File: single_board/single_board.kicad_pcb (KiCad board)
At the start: 4 copper layers, 118.6 x 108.9 mm, 121 parts, among them J1 SWD, J11 SPI Debug, J17 BOOTSEL, J2 USB_C_Receptacle_USB2.0_16P, J3 RST, J30 JST_GH_H, J31 JST_GH_H, J32 PB_Vertical, J33 JST_GH_H, J34 PB_Vertical, J35 JST_GH_H, J36 JST_GH_H, J37 JST_GH_H, J38 PB_Vertical, J39 PB_Vertical, J4 Conn_01x02, J40 PB_Vertical, J41 PB_Vertical, J42 PB_Vertical, J43 PB_Vertical, J44 PB_Vertical, J45 PB_Vertical, J46 PB_Vertical, J47 PB_Vertical, J48 PB_Vertical, J49 PB_Vertical, J5 Conn_01x02, J50 PB_Vertical, J6 Conn_01x02, J7 Conn_01x02, Q1 AO3401A, Q2 AO3401A, Q3 AO3401A, Q4 AO3401A, Q5 2N7002, SW1 Button, U1 AP2112K-3.3, U3 USBLC6-2SC6, U4 LSM6DSV, U5 STM32G474VBTx, Y1 FC-135

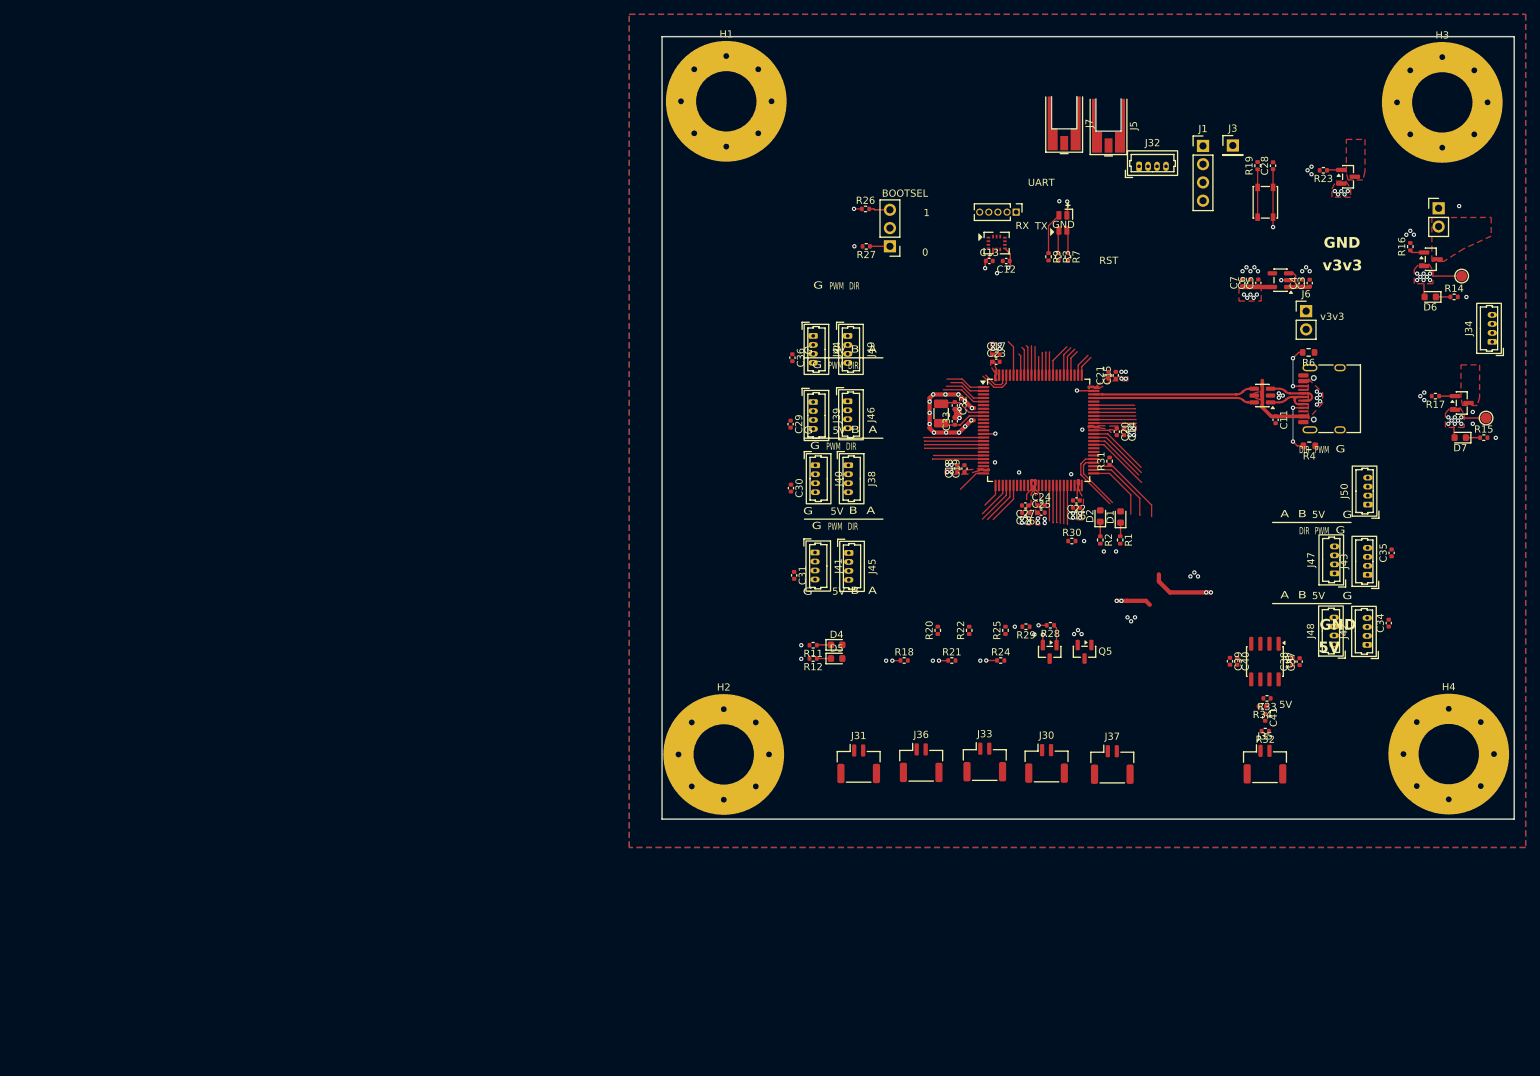
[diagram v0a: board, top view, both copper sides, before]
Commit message: PCB Layout
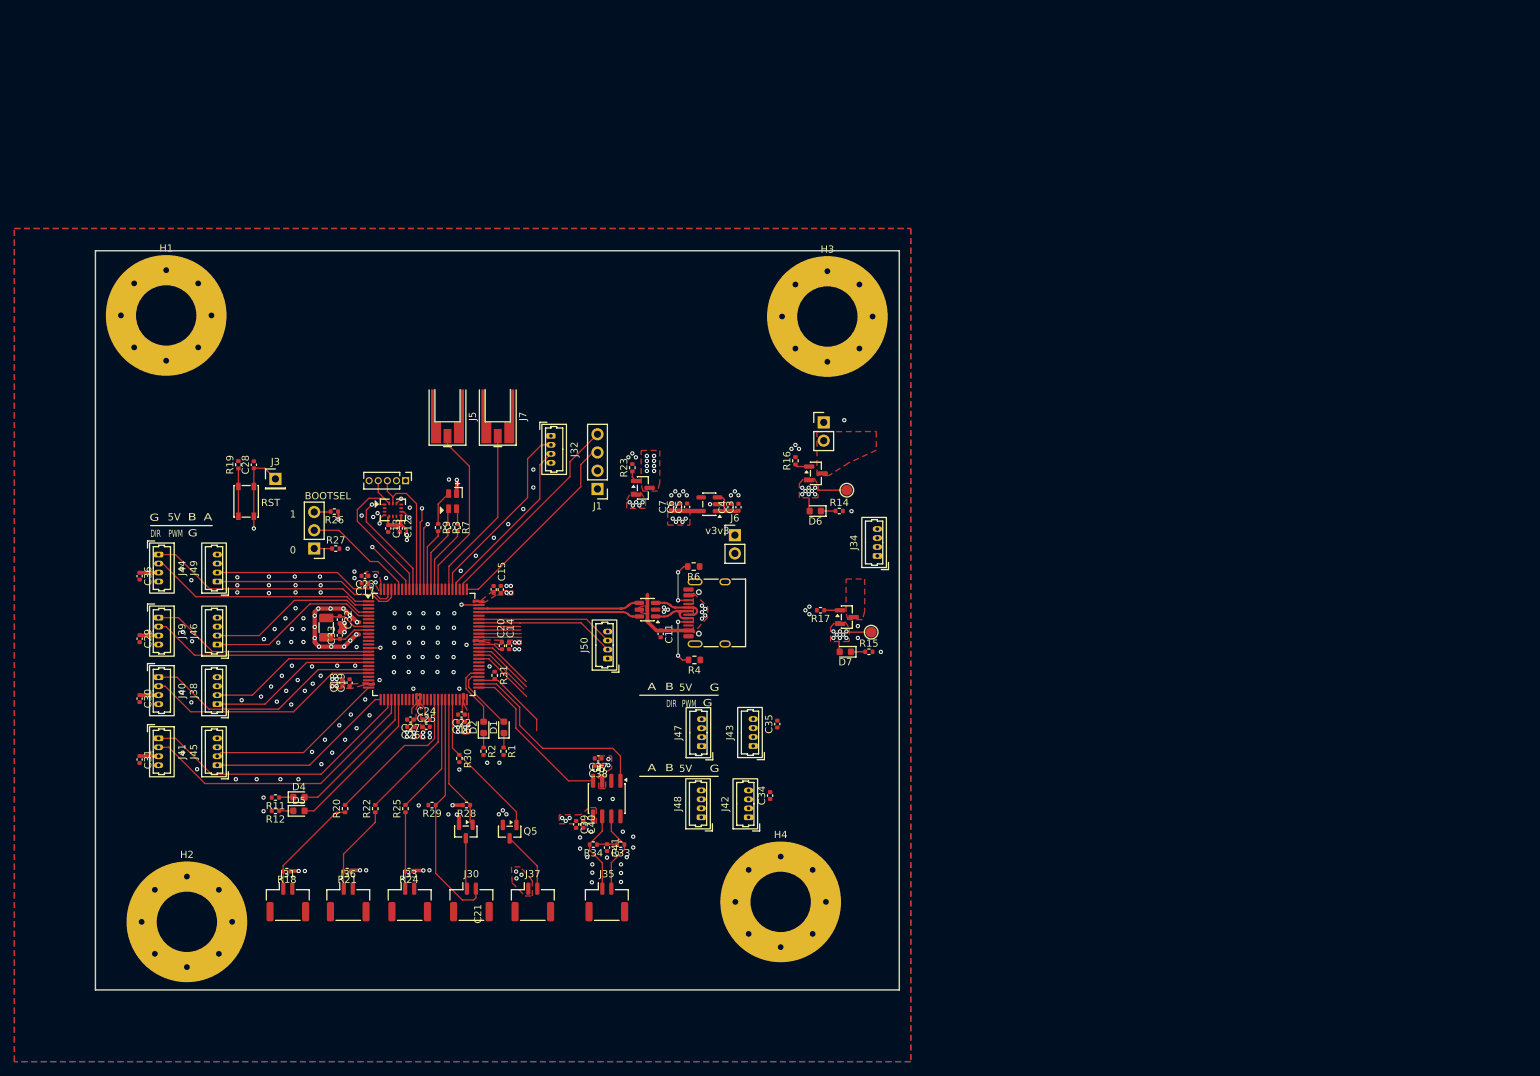
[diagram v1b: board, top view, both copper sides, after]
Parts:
- removed R32: 120, Resistor_SMD:R_0402_1005Metric
- moved C28 147.8 mm to (40.8, 118.8)
- moved R19 147.8 mm to (38.6, 118.8)
- moved SW1 147.8 mm to (39.7, 123.9)
- moved J3 141.1 mm to (43.8, 120.8)
- moved J50 107.9 mm to (90.0, 145.8)
- moved Q3 107.3 mm to (94.9, 122.0)
- moved R23 104.7 mm to (93.5, 119.2), turned to 90 degrees
- moved J5 100.5 mm to (67.8, 112.1)
- moved C37 98.6 mm to (88.7, 159.7), turned to 180 degrees
- moved C38 97.7 mm to (88.7, 160.7), turned to 180 degrees
- moved J1 96.9 mm to (88.6, 122.2), turned to 180 degrees
- moved J44 96.0 mm to (27.6, 131.3)
- moved J40 96.0 mm to (27.5, 148.4)
- moved J39 95.9 mm to (27.6, 140.1)
- moved C36 95.8 mm to (24.9, 134.3)
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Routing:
- net /ENC3_B: track 6.06 -> 40.4 mm
- net /ENC3_A: track 5.11 -> 38.9 mm
- net /RST: track 9.65 -> 42.3 mm
- net /FSR_ADC: track 5.26 -> 33.3 mm
- net /ENC6_B: track 5.01 -> 31.6 mm
- net /ENC2_A: track 6.90 -> 33.3 mm
- net /ENC6_A: track 5.57 -> 31.9 mm
- net /SWCLK: track 3.33 -> 29.3 mm
- net /ENC2_B: track 7.10 -> 32.9 mm
- net /SWDIO: track 2.99 -> 27.9 mm
- net /DIR2: track 3.35 -> 26.5 mm
- net /ENC1_A: track 8.30 -> 31.2 mm
- net /ENC1_B: track 8.20 -> 30.9 mm
- net /UART4_RX: track 4.04 -> 26.5 mm
- net /PWM6: track 4.10 -> 26.4 mm
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- added copper zone on In2.Cu, net /v3v3IN_debug
- removed copper zone on In2.Cu, net 5V
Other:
- board size 118.6 x 108.9 mm -> 111.9 x 102.9 mm
- board text removed: "GND"
- board text removed: "RX"
- board text removed: "TX"
- board text removed: "UART"
